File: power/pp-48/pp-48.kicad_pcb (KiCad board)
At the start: 4 copper layers, 50 x 72 mm, 110 parts, among them J101 NODE 19V, J102 FRONT PANEL, J103 AUX, J201 NODE 19V, J202 FRONT PANEL, J203 AUX, Q101 BSC070N10NS5, Q102 2N7002, Q103 2N7002, Q104 2N7002, Q105 2N7002, Q201 BSC070N10NS5, Q202 2N7002, Q203 2N7002, Q204 2N7002, Q205 2N7002, U101 LM5069MM-2, U102 INA238AIDGSR, U103 74LVC1G74, U104 ADC121C027CIMK, U105 TCA9535PWR, U106 TLP176AM, U107 TLP176AM, U108 TLP291, U201 LM5069MM-2, U202 INA238AIDGSR, U203 74LVC1G74, U204 ADC121C027CIMK, U205 TCA9535PWR, U206 TLP176AM, U207 TLP176AM, U208 TLP291

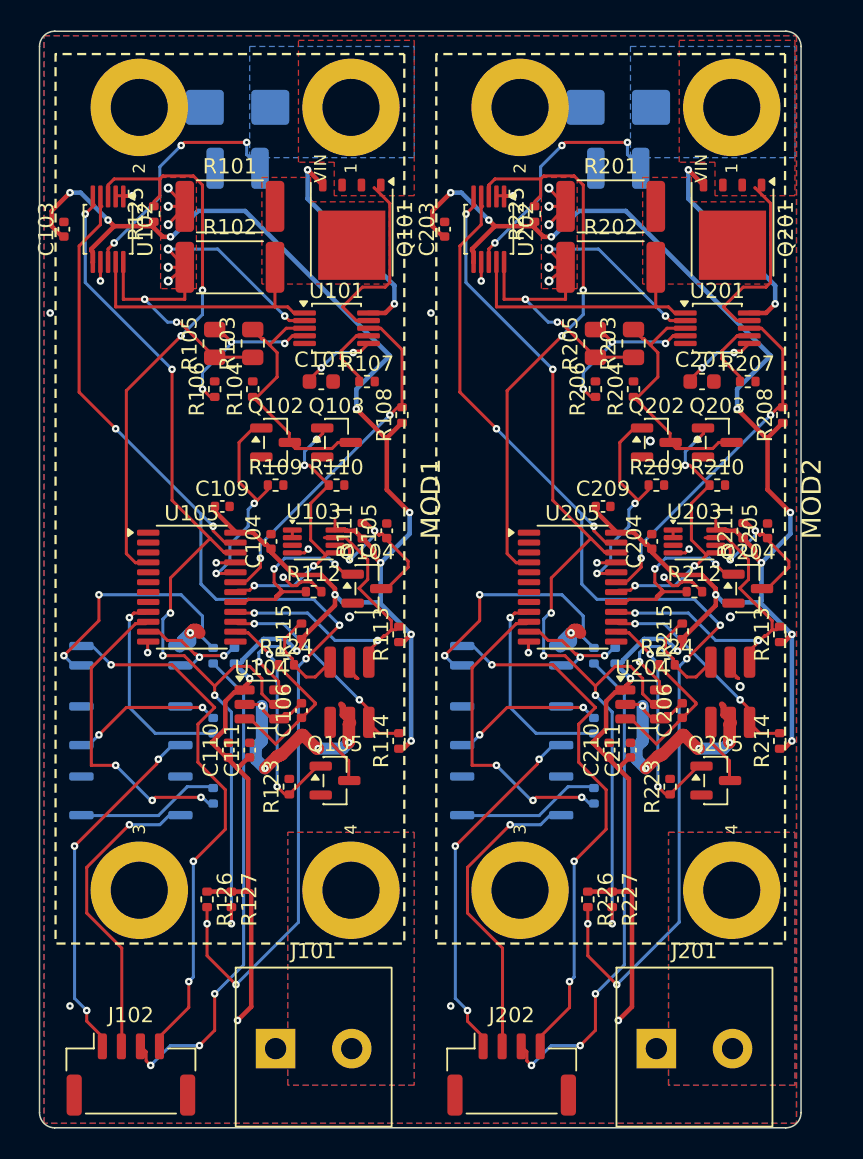
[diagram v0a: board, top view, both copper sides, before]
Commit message: pp-48: DRC clean: solid connections on the starved GND pads, U3 +3V3 router stub removed, last column's +3V3 trunk ends at its tap, module outline Fab only on the plane (pmmount host_outline(silk=False)), silk tidied; core-side channel / trunk ends stored as DRC exclusions until the core is drawn; handoff
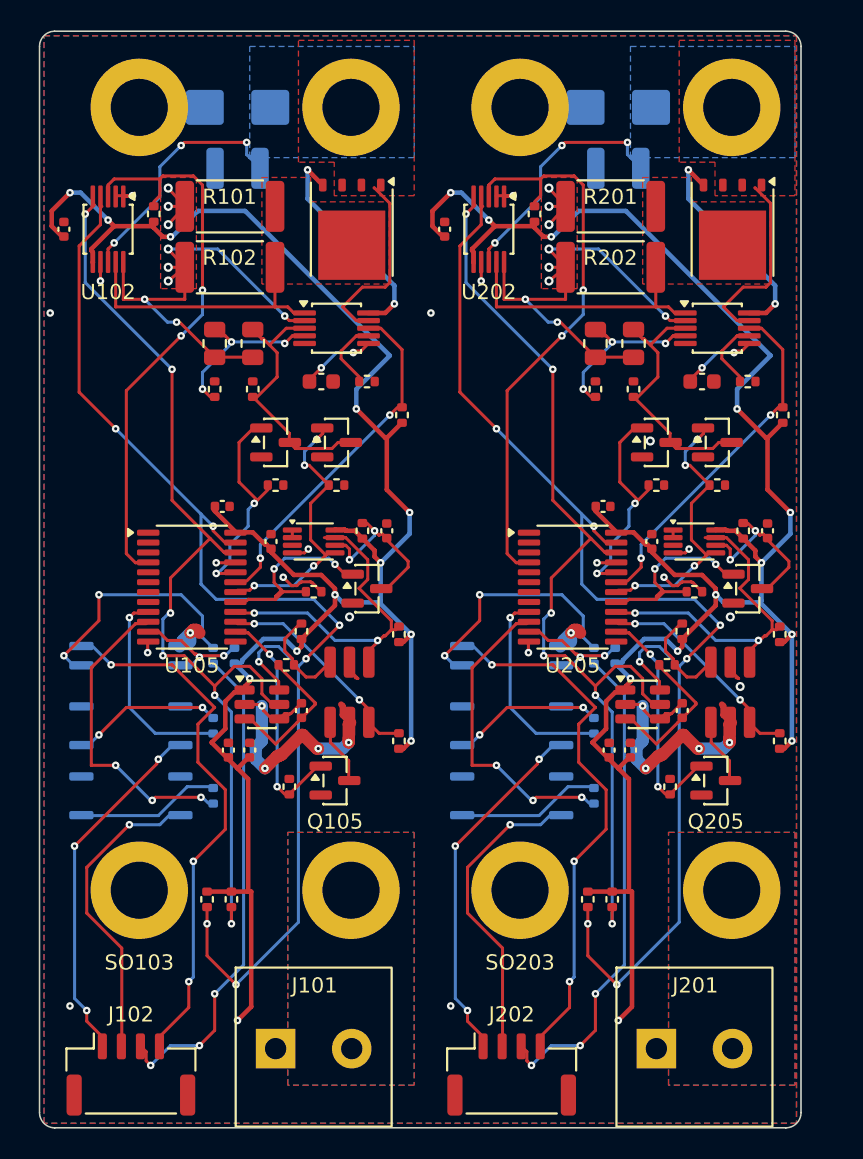
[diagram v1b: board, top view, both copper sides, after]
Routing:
- net +3V3: track 301.6 -> 288.9 mm
